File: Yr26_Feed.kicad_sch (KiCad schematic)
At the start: 13 parts

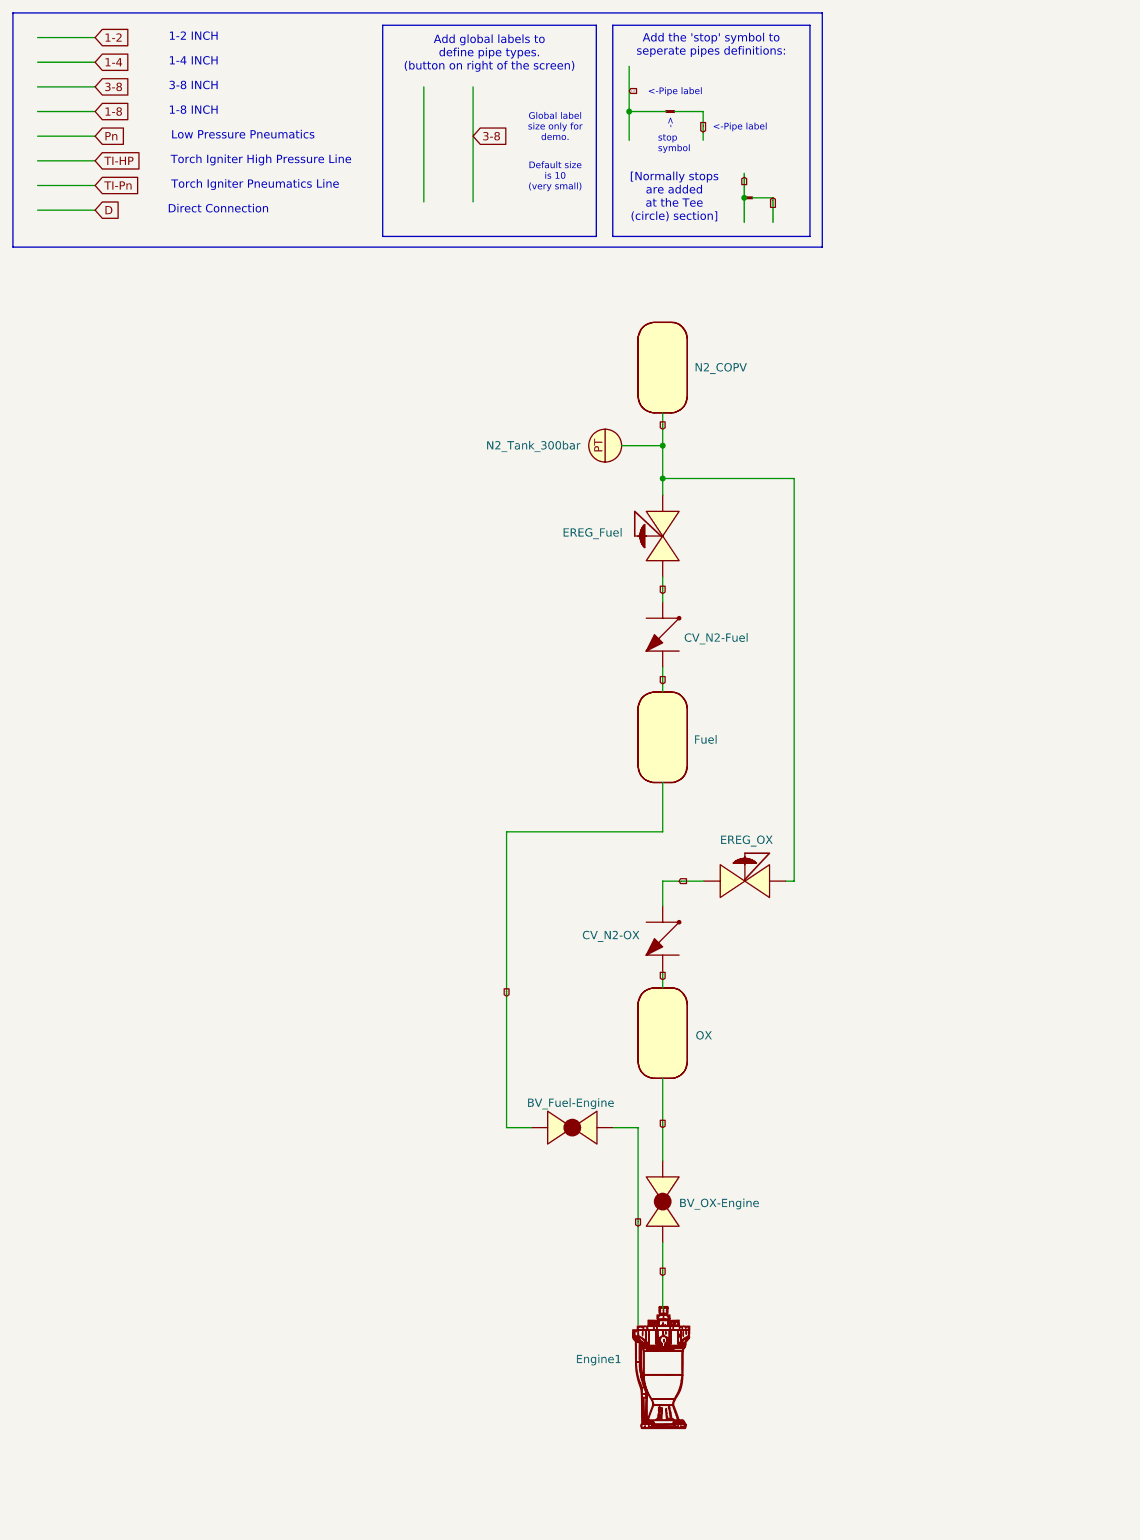
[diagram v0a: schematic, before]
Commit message: Feed System Ver 1
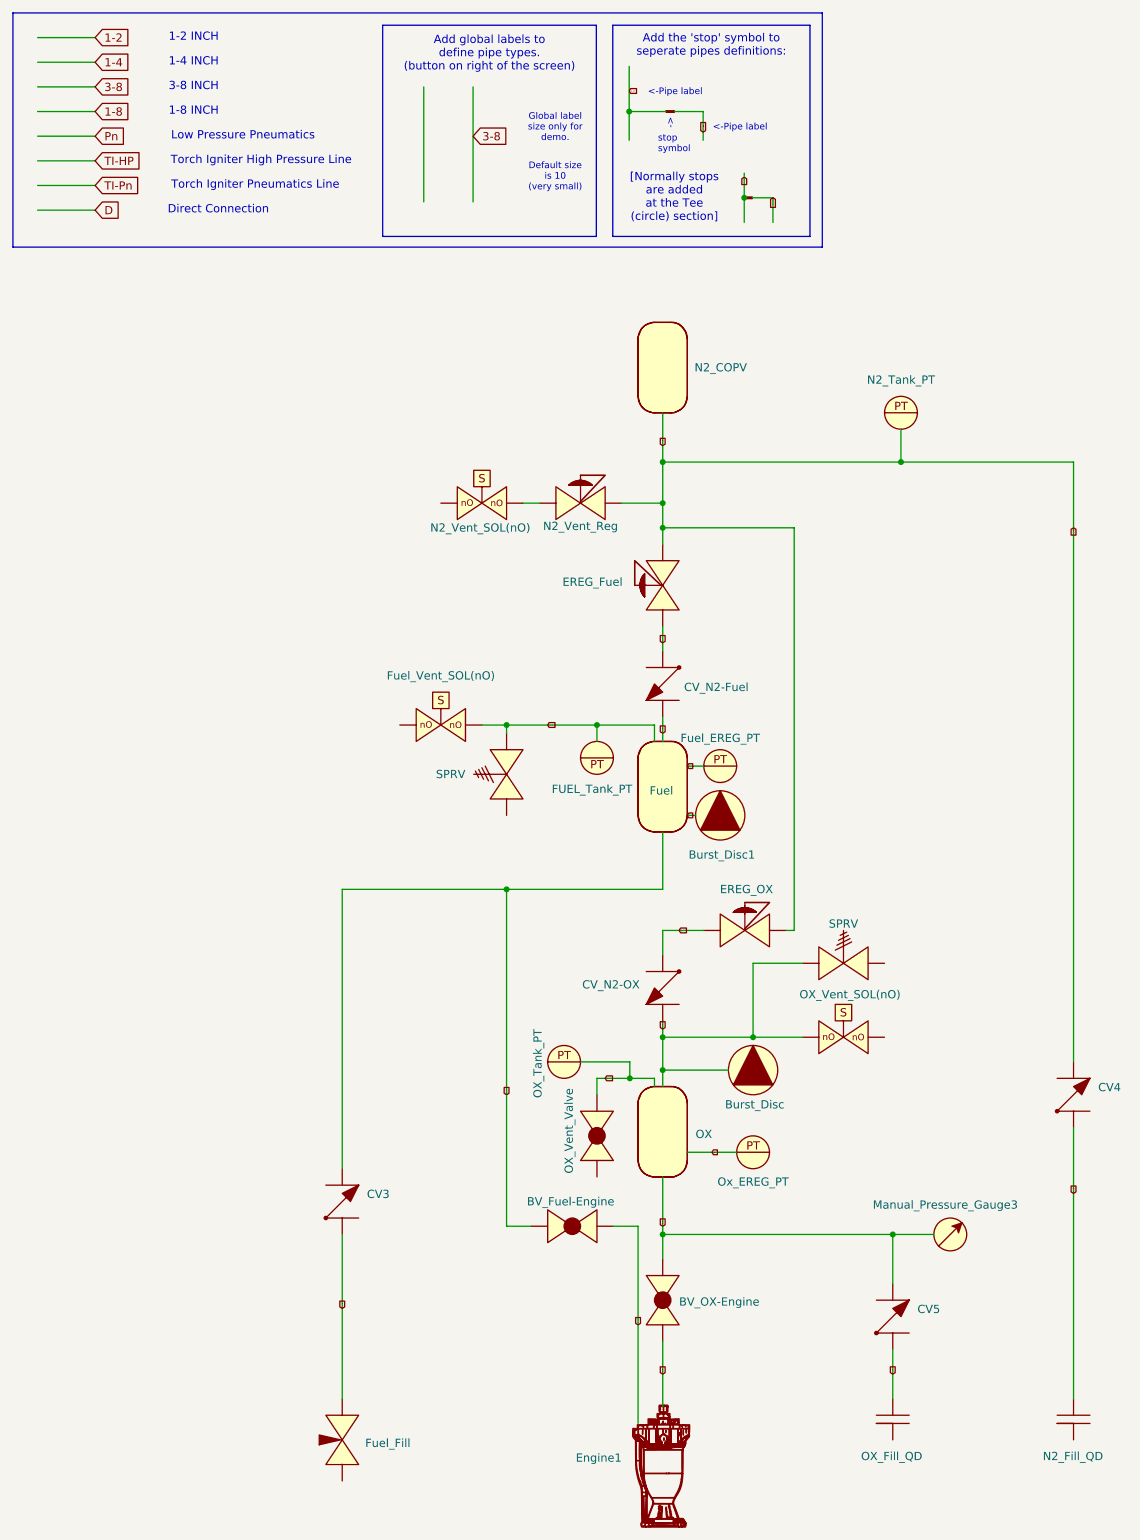
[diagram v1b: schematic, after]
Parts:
- removed N2_Tank_300bar: ~, symbol PID_symbols:Pressure_Transducer
- added Burst_Disc, Burst_Disc1: ~, symbol PID_symbols:Burst_Disc
- added CV3, CV4, CV5: ~, symbol PID_symbols:Check_Valve
- added FUEL_Tank_PT, Fuel_EREG_PT, N2_Tank_PT, OX_Tank_PT, Ox_EREG_PT: ~, symbol PID_symbols:Pressure_Transducer
- added Fuel_Fill: ~, symbol PID_symbols:Needle_Valve
- added Fuel_Vent_SOL(nO), N2_Vent_SOL(nO), OX_Vent_SOL(nO): ~, symbol PID_symbols:Normally Open Solenoid
- added Manual_Pressure_Gauge3: ~, symbol PID_symbols:Manual_Pressure_Gauge
- added N2_Fill_QD, OX_Fill_QD: ~, symbol PID_symbols:Quick_Disconnect
- added N2_Vent_Reg: ~, symbol PID_symbols:Pressure_Regulator
- added OX_Vent_Valve: ~, symbol PID_symbols:Ball_Valve
- added SPRV (x2): ~, symbol PID_symbols:SPRV
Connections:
- net 1-2: now also CV3.
- net 1-4: now also Burst_Disc., CV3., CV4., CV5., FUEL_Tank_PT., Fuel_Fill., Fuel_Vent_SOL(nO)., N2_Fill_QD., N2_Tank_PT., N2_Vent_Reg., OX_Fill_QD., OX_Tank_PT., OX_Vent_SOL(nO)., OX_Vent_Valve., SPRV., SPRV.
- net 3-4: now also CV5., Manual_Pressure_Gauge3.
- net D: now also Burst_Disc1., Fuel_EREG_PT., Ox_EREG_PT.
- new net: N2_Vent_Reg., N2_Vent_SOL(nO).
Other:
- moved on the sheet: BV_Fuel-Engine, BV_OX-Engine, CV_N2-Fuel, CV_N2-OX, EREG_Fuel, EREG_OX, Engine1, Fuel, OX
